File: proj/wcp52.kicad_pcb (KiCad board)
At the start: 4 copper layers, 100 x 100 mm, 301 parts, among them J1 MicroUSB-B, J2 IN1, J3 IN2, J4 OUT, Q1 MMBT3906, Q10 MMBT3904, Q11 BFR540, Q12 BFR540, Q13 MMBT3904, Q14 MMBT3904, Q15 MMBT3904, Q16 MMBT3904, Q17 PZT2907A, Q18 PZT2907A, Q19 MMBT3904, Q2 IRLML6402, Q3 AOD417, Q4 MMBT3906, Q5 2N7002, Q6 2N7002, Q7 MMBT3906, Q8 2N7002, Q9 2N7002, U1 TL431AIDBZ, U10 MASWSS0162, U11 AD8310ARMZ, U12 ATSAM4S16CA-AU, U13 FT230XS, U14 L78M05CDT, U15 MC79M05CDT, U16 AZ1117CH-1.8TRG1, U17 MCP1700T-vv02E/TT, U2 LM393M, U3 LMH6714MF, U4 AD9958BCPZ, U5 LMH6714MF, U6 AD8000YRDZ, U7 THS3001IDGN, U8 MAADSS0008, U9 MASWSS0162, X1 25 MHz, X2 12MHz

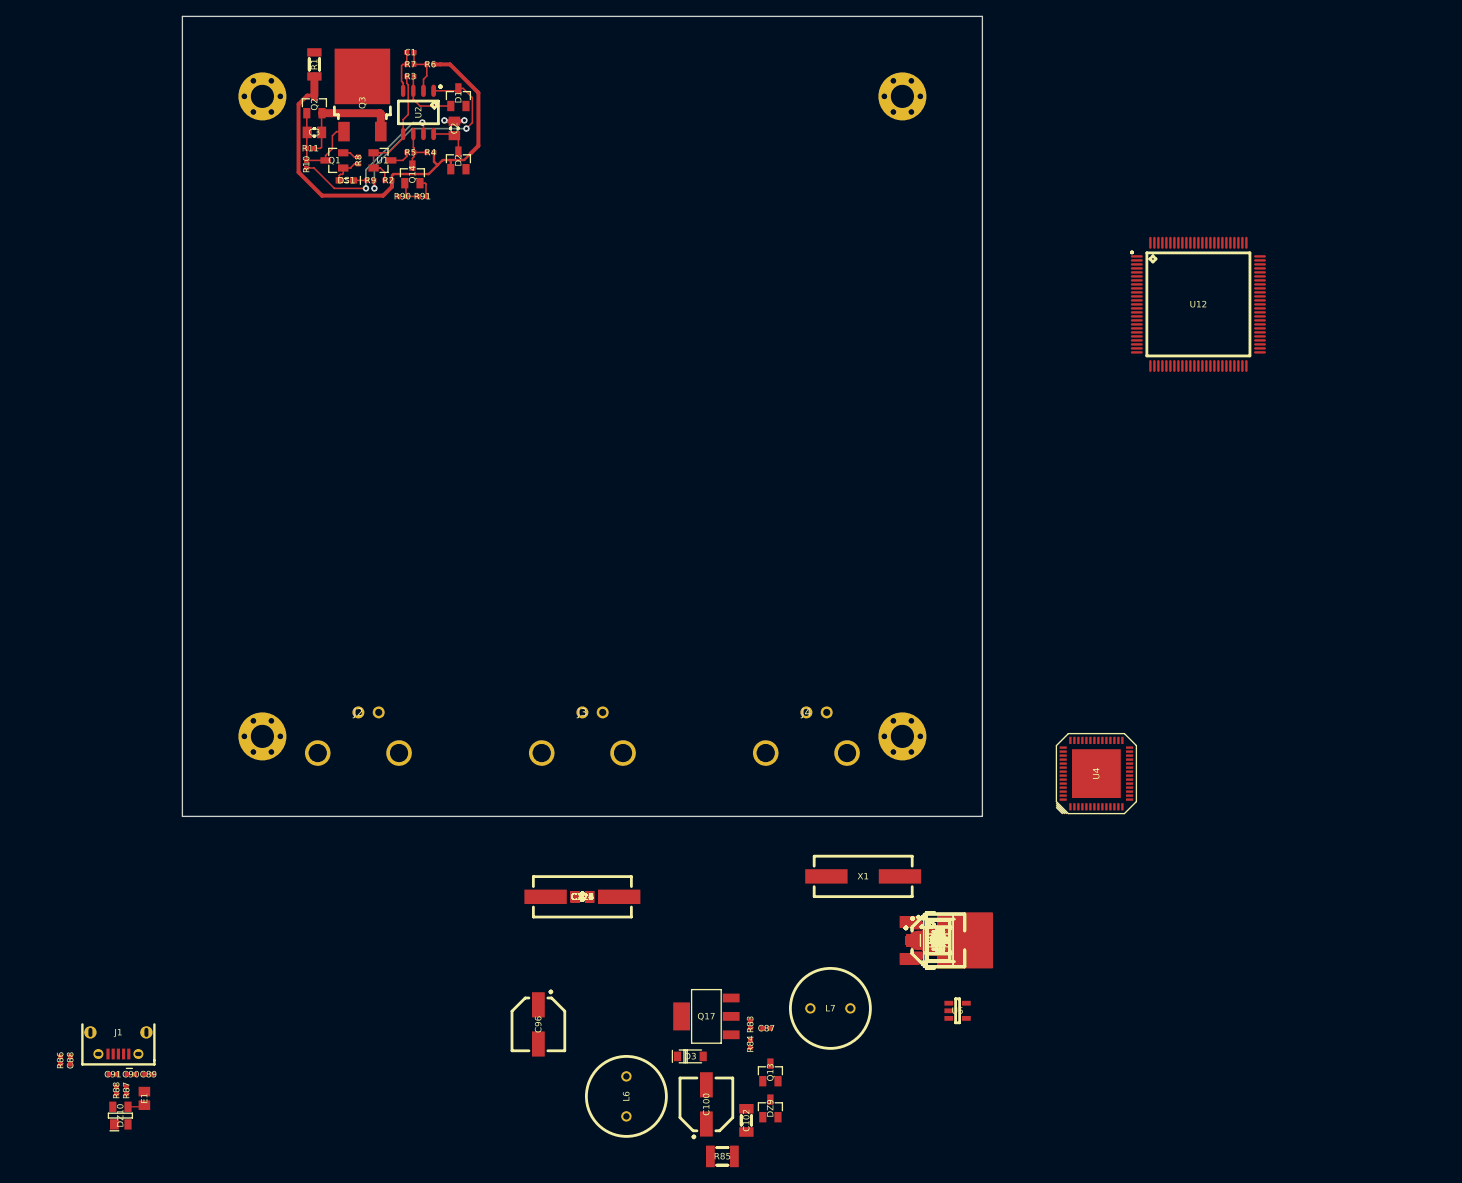
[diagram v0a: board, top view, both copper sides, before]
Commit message: Layout most analog bits
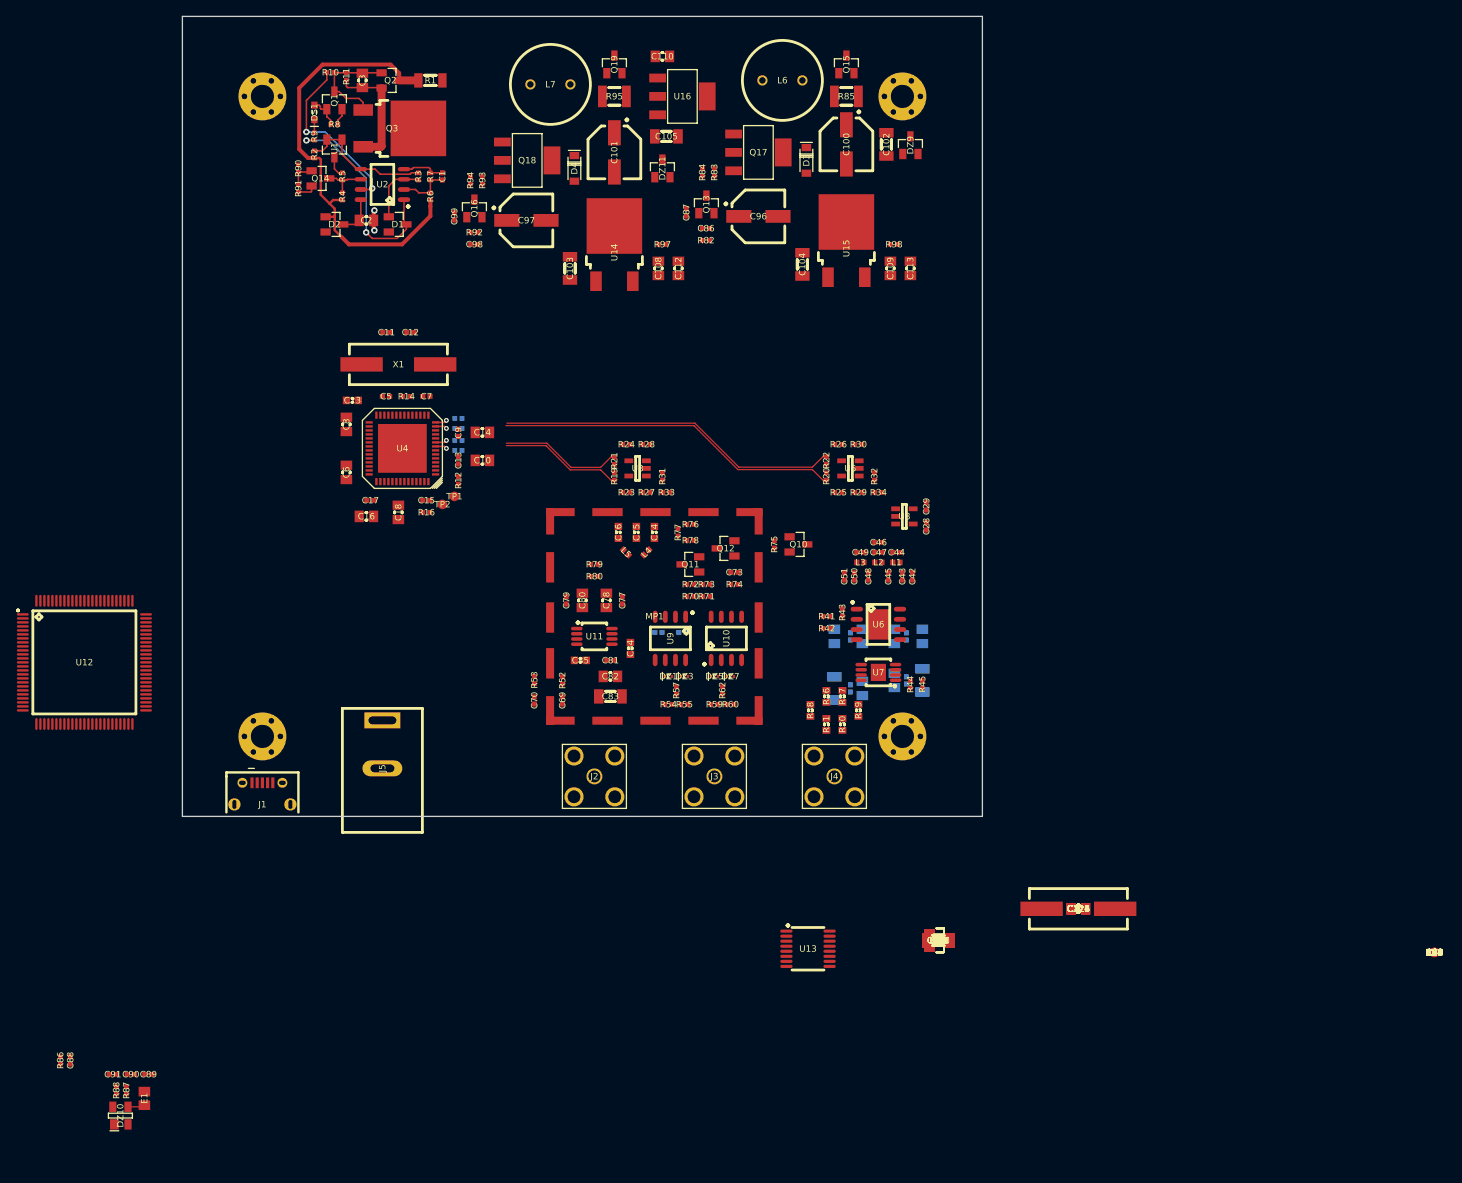
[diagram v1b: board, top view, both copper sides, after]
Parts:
- added J5: CONN-PJ-037A, conn-cui:CONN-PJ-037A, F.Cu at (100.0, 119.0)
- added MP1: SHIELD, manuf:LAIRD-BMI-S-203, F.Cu at (134.0, 100.0)
- C30, C31, C32, C33, C34, C35, C36, C37, C38, C39, C40, C41, C71, C72, R13, R15, R17, R18: moved to B.Cu
- J2, J3, J4: footprint manuf:CONN-BNC-1-1337543-0 -> manuf:CONN-TE-1814400
- moved U12 146.3 mm to (62.8, 105.8)
- moved R85 133.4 mm to (158.0, 35.0)
- moved L6 128.5 mm to (150.0, 33.0), turned to 180 degrees
- moved C102 123.2 mm to (163.0, 41.0), turned to 270 degrees
- moved DZ9 121.7 mm to (166.0, 41.1)
- moved C100 121.3 mm to (158.0, 41.0), turned to 270 degrees
- moved L7 120.7 mm to (121.0, 33.5), turned to 180 degrees
- moved Q19 116.8 mm to (129.0, 31.0), turned to 90 degrees
- moved C110 115.8 mm to (135.0, 30.0), turned to 180 degrees
- moved R95 113.0 mm to (129.0, 35.0), turned to 180 degrees
- moved D3 112.9 mm to (153.0, 43.0), turned to 270 degrees
- moved R94 111.6 mm to (111.0, 45.5), turned to 270 degrees
- moved R93 110.8 mm to (112.5, 45.5), turned to 90 degrees
- moved U16 110.3 mm to (137.5, 35.0)
- moved Q18 110.2 mm to (118.1, 43.0)
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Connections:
- U8 pad 2: Net-(U8-Pad2) -> GND
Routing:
- net /Synth/CH1_P: track 0.00 -> 44.3 mm, vias 0 -> 1
- net /Synth/CH1_N: track 0.00 -> 44.2 mm, vias 0 -> 1
- net /Synth/CH0_N: track 0.00 -> 16.7 mm, vias 0 -> 1
- net /Synth/CH0_P: track 0.00 -> 16.7 mm, vias 0 -> 1
